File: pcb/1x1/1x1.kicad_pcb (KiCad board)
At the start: 2 copper layers, 5 parts, among them J1 Conn_02x04_Odd_Even, SW1 SW_Push

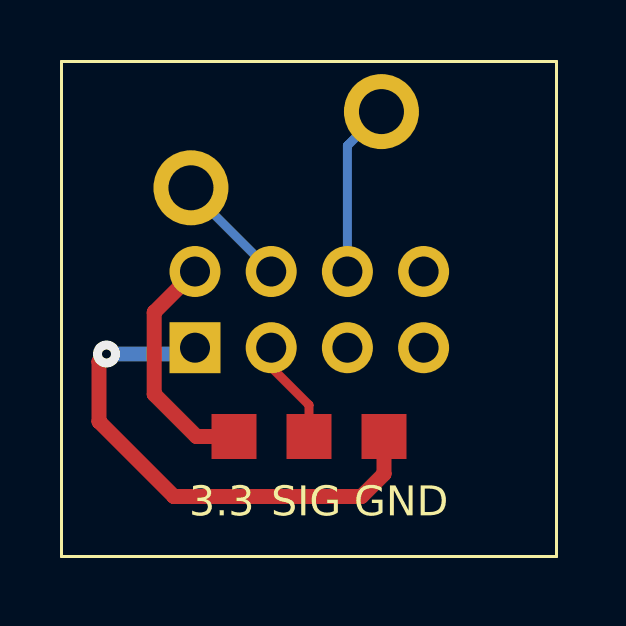
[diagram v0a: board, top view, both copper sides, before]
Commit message: pcb 1x1 sync
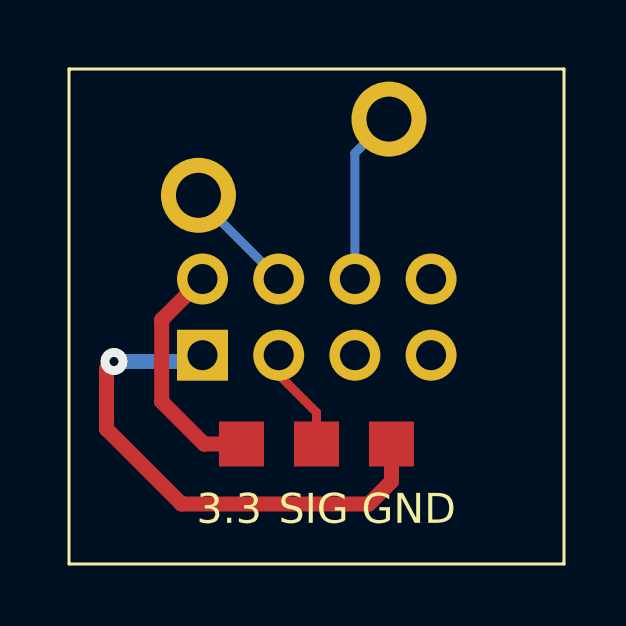
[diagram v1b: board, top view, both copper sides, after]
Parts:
- moved J1 0.35 mm to (4.45, 9.54)
- moved SW1 0.35 mm to (8.12, 6.75)
- moved TP1 0.35 mm to (8.25, 12.5)
- moved TP2 0.35 mm to (10.8, 12.5)
- moved TP3 0.35 mm to (5.75, 12.5)
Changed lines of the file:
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@@
 	(footprint "TestPoint:TestPoint_Pad_1.5x1.5mm"
 		(layer "F.Cu")
-		(at 10.5 12.25)
+		(at 10.75 12.5)
 		(descr "SMD rectangular pad as test Point, square 1.5mm side length")
 		(tags "test point SMD pad rectangle square")
@@
 	(footprint "TestPoint:TestPoint_Pad_1.5x1.5mm"
 		(layer "F.Cu")
-		(at 5.5 12.25)
+		(at 5.75 12.5)
 		(descr "SMD rectangular pad as test Point, square 1.5mm side length")
 		(tags "test point SMD pad rectangle square")
@@
 	(footprint "TestPoint:TestPoint_Pad_1.5x1.5mm"
 		(layer "F.Cu")
-		(at 8 12.25)
+		(at 8.25 12.5)
 		(descr "SMD rectangular pad as test Point, square 1.5mm side length")
 		(tags "test point SMD pad rectangle square")
@@
 	(footprint "PCM_Switch_Keyboard_Cherry_MX:SW_Cherry_MX_Plate"
 		(layer "F.Cu")
-		(at 7.875 6.5)
+		(at 8.125 6.75)
 		(descr "Cherry MX keyswitch Plate Mount")
 		(tags "Cherry MX Keyboard Keyswitch Switch Plate Cutout")
@@
 	)
 	(footprint "Connector_PinSocket_2.54mm:PinSocket_2x04_P2.54mm_Vertical"
-		(locked yes)
 		(layer "B.Cu")
-		(at 4.2 9.29 -90)
+		(at 4.45 9.54 -90)
 		(descr "Through hole straight socket strip, 2x04, 2.54mm pitch, double cols (from Kicad 4.0.7), script generated")
 		(tags "Through hole socket strip THT 2x04 2.54mm double row")
@@
 	)
 	(gr_rect
-		(start -0.25 -0.25)
-		(end 16.25 16.25)
-		(locked yes)
+		(start 0 0)
+		(end 16.5 16.5)
 		(stroke
 			(width 0.1)
@@
 		(layer "F.SilkS")
 	)
-	(gr_rect
-		(start 4.25 15.5)
-		(end 11.75 17.5)
-		(stroke
-			(width 0.15)
-			(type default)
-		)
-		(fill none)
-		(layer "Dwgs.User")
-	)
-	(gr_line
-		(start 10.5 12.5)
-		(end 10.5 15.5)
-		(stroke
-			(width 0.8)
-			(type default)
-		)
-		(layer "Dwgs.User")
-	)
-	(gr_line
-		(start 5.5 12.5)
-		(end 5.5 15.5)
-		(stroke
-			(width 0.8)
-			(type default)
-		)
-		(layer "Dwgs.User")
-	)
-	(gr_line
-		(start 8 12.5)
-		(end 8 15.5)
-		(stroke
-			(width 0.8)
-			(type default)
-		)
-		(layer "Dwgs.User")
-	)
 	(gr_text "3.3"
-		(at 4 15 0)
+		(at 4.25 15.25 0)
 		(layer "F.SilkS")
 		(effects
@@
 	)
 	(gr_text "SIG"
-		(at 6.735715 15 0)
+		(at 6.985715 15.25 0)
 		(layer "F.SilkS")
 		(effects
@@
 	)
 	(gr_text "GND"
-		(at 9.5 15 0)
+		(at 9.75 15.25 0)
 		(layer "F.SilkS")
 		(effects
@@
 	)
 	(segment
-		(start 6.74 6.75)
-		(end 4.065 4.075)
+		(start 6.99 7)
+		(end 4.315 4.325)
 		(width 0.3)
 		(layer "B.Cu")
@@
 	)
 	(segment
-		(start 4.065 4.075)
-		(end 4.065 3.96)
+		(start 4.315 4.325)
+		(end 4.315 4.21)
 		(width 0.3)
 		(layer "B.Cu")
@@
 	)
 	(segment
-		(start 9.28 6.75)
-		(end 9.28 2.555)
+		(start 9.53 7)
+		(end 9.53 2.805)
 		(width 0.3)
 		(layer "B.Cu")
@@
 	)
 	(segment
-		(start 9.28 2.555)
-		(end 10.415 1.42)
+		(start 9.53 2.805)
+		(end 10.665 1.67)
 		(width 0.3)
 		(layer "B.Cu")
@@
 	)
 	(segment
-		(start 8 11.2)
-		(end 6.74 9.94)
+		(start 8.25 11.45)
+		(end 6.99 10.19)
 		(width 0.3)
 		(layer "F.Cu")
@@
 	)
 	(segment
-		(start 6.74 9.94)
-		(end 6.74 9.29)
+		(start 6.99 10.19)
+		(end 6.99 9.54)
 		(width 0.3)
 		(layer "F.Cu")
@@
 	)
 	(segment
-		(start 8 12.25)
-		(end 8 11.2)
+		(start 8.25 12.5)
+		(end 8.25 11.45)
 		(width 0.3)
 		(layer "F.Cu")
@@
 	)
 	(segment
-		(start 9.75 14.25)
-		(end 3.5 14.25)
+		(start 10 14.5)
+		(end 3.75 14.5)
 		(width 0.5)
 		(layer "F.Cu")
@@
 	)
 	(segment
-		(start 10.5 12.25)
-		(end 10.5 13.5)
+		(start 10.75 12.5)
+		(end 10.75 13.75)
 		(width 0.5)
 		(layer "F.Cu")
@@
 	)
 	(segment
-		(start 10.5 13.5)
-		(end 9.75 14.25)
+		(start 10.75 13.75)
+		(end 10 14.5)
 		(width 0.5)
 		(layer "F.Cu")
@@
 	)
 	(segment
-		(start 1 9.75)
-		(end 1.25 9.5)
+		(start 1.25 10)
+		(end 1.5 9.75)
 		(width 0.5)
 		(layer "F.Cu")
@@
 	)
 	(segment
-		(start 3.5 14.25)
-		(end 1 11.75)
+		(start 3.75 14.5)
+		(end 1.25 12)
 		(width 0.5)
 		(layer "F.Cu")
@@
 	)
 	(segment
-		(start 1 11.75)
-		(end 1 9.75)
+		(start 1.25 12)
+		(end 1.25 10)
 		(width 0.5)
 		(layer "F.Cu")
@@
 	)
 	(via
-		(at 1.25 9.5)
+		(at 1.5 9.75)
 		(size 0.9)
 		(drill 0.3)
@@
 	)
 	(segment
-		(start 1.25 9.5)
-		(end 3.99 9.5)
+		(start 1.5 9.75)
+		(end 4.24 9.75)
 		(width 0.5)
 		(layer "B.Cu")
@@
 	)
 	(segment
-		(start 3.99 9.5)
-		(end 4.2 9.29)
+		(start 4.24 9.75)
+		(end 4.45 9.54)
 		(width 0.5)
 		(layer "B.Cu")
@@
 	)
 	(segment
-		(start 5.5 12.25)
-		(end 4.25 12.25)
+		(start 5.75 12.5)
+		(end 4.5 12.5)
 		(width 0.5)
 		(layer "F.Cu")
@@
 	)
 	(segment
-		(start 2.84 10.84)
-		(end 2.84 8.11)
+		(start 3.09 11.09)
+		(end 3.09 8.36)
 		(width 0.5)
 		(layer "F.Cu")
@@
 	)
 	(segment
-		(start 4.25 12.25)
-		(end 2.84 10.84)
+		(start 4.5 12.5)
+		(end 3.09 11.09)
 		(width 0.5)
 		(layer "F.Cu")
@@
 	)
 	(segment
-		(start 2.84 8.11)
-		(end 4.2 6.75)
+		(start 3.09 8.36)
+		(end 4.45 7)
 		(width 0.5)
 		(layer "F.Cu")
 		(net 8)
 	)
+	(group ""
+		(members "0c135175-a099-48ac-aeba-853512bca50d" "22e562be-d6c2-4592-8d6b-d5240938552e"
+			"230cbc67-778c-4747-98ef-4b8a575b3398" "2b83875f-453e-44f2-9988-29eec695e375"
+			"3b1defd3-6595-473b-afde-936d988cae9c" "3bd26f5c-1151-4bca-8395-a38191cb26ae"
+			"4be51fed-9d2f-488c-bb78-5551fc454827" "538e550a-a875-44da-b286-aef072ebb876"
+			"65673f39-d3a2-4c85-aec4-16f97a4185f6" "66eb1448-f2e7-4207-b76b-20a3aaae2fc6"
+			"6a1d5882-8d63-4011-80a3-e4a25d5b9969" "72727f99-f366-4272-9d34-113b196e64d7"
+			"8898c26a-8a30-43f4-9542-f7835620852d" "a29d0cfb-4d49-41a3-bbb5-6166698eda8e"
+			"a6ebf16b-ec2c-482c-a5b5-78447953d043" "b1e3ab74-68b0-4c02-9135-86217cdf91d2"
+			"b33b61e3-8756-4f59-a425-10eec9bb35d7" "b5839378-041c-43a3-aa09-18a0f17fbd7f"
+			"c671fe42-9d5e-4d41-b245-7dbfd924746c" "c93ff858-25ec-495a-9ee4-a07c55a42d0f"
+			"cee5d891-e317-4017-8582-2736ff02497e" "cf40a6c9-04c6-4921-ae18-34d4edf9ce7d"
+			"d40d1ecf-1d2c-4e51-a97f-919b4ccaaf98" "d98f1aac-ff58-4e9f-9ef8-f28ab99bf7cb"
+			"dbd6544a-9e52-4290-abd9-5e3f4f779e36" "dc11ac07-0243-4b52-9fcc-7a6ec4d11fe6"
+			"e2d1d1e6-76f8-423a-a01d-994193155227" "eaaa80f7-0dd7-49d8-9fa1-d3dd4181ccf6"
+			"fd66a5b7-c19c-4e5f-8396-97fd9fefa0bb"
+		)
+	)
 )
